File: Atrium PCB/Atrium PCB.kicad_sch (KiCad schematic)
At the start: 167 parts, among them J1 Conn_01x05_Pin, SW1 EC11E09244BS, SW10 SW_Push, SW11 SW_Push, SW12 SW_Push, SW13 SW_Push, SW14 SW_Push, SW15 SW_Push, SW16 SW_Push, SW17 SW_Push, SW18 SW_Push, SW19 SW_Push, SW2 SKRPACE010, SW20 SW_Push, SW21 SW_Push, SW22 SW_Push, SW23 SW_Push, SW24 SW_Push, SW25 SW_Push, SW26 SW_Push, SW27 SW_Push, SW28 SW_Push, SW29 SW_Push, SW3 SKRPACE010, SW30 SW_Push, SW31 SW_Push, SW32 SW_Push, SW33 SW_Push, SW34 SW_Push, SW35 SW_Push, SW36 SW_Push, SW37 SW_Push, SW38 SW_Push, SW39 SW_Push, SW4 SW_Push, SW40 SW_Push, SW41 SW_Push, SW42 SW_Push, SW43 SW_Push, SW44 SW_Push, SW45 SW_Push, SW46 SW_Push, SW47 SW_Push, SW48 SW_Push, SW49 SW_Push, SW5 SW_Push, SW6 SW_Push, SW7 SW_Push, SW8 SW_Push, SW9 SW_Push, U12 AP2112K-3.3, U4 SN74LVC1T45DBVR, X1 X322512MSB4SI

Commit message: sync
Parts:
- removed C44, C46, C47, C48: 100nF, Capacitor_SMD:C_0603_1608Metric, symbol Device:C
- removed C45: 10uF, Capacitor_SMD:C_0805_2012Metric, symbol Device:C
- removed D10, D15, D19, D23, D27, D31, D35, D39, D4: D, symbol Device:D
- removed LED10, LED7, LED8, LED9: SK6812MINI-E_C5149201, easyeda2kicad:LED-SMD_4P-L3.2-W2.8-LS5.9_SK6812MINI-E, symbol easyeda2kicad:SK6812MINI-E_C5149201
- removed R19, R9: 470, Resistor_SMD:R_0603_1608Metric, symbol Device:R
- removed SW12, SW17, SW21, SW25, SW29, SW33, SW37, SW41, SW7: SW_Push, symbol Switch:SW_Push
- removed U4: SN74LVC1T45DBVR, easyeda2kicad:SOT-23-6_L2.9-W1.6-P0.95-LS2.8-BR, symbol easyeda2kicad:SN74LVC1T45DBVR
- added C100, C101, C102, C103, C104, C105, C106, C107, C108, C109, C110, C111, C112, C113, C114, C115, C116, C117, C118, C119, C120, C121, C122, C123, C124, C125, C126, C127, C128, C129, C130, C131, C132, C133, C134, C135, C136, C137, C138, C139, C140, C141, C142, C143, C144, C145, C146, C147, C148, C149, C150, C151, C152, C153, C154, C155, C156, C157, C158, C159, C160, C161, C162, C163, C164, C165, C166, C167, C168, C169, C170, C171, C172, C173, C174, C175, C176, C177, C178, C179, C180, C181, C182, C183, C184, C185, C186, C187, C188, C189, C190, C191, C192, C193, C194, C195, C196, C197, C198, C199, C200, C201, C202, C203, C204, C205, C206, C207, C208, C209, C210, C217, C218, C219, C220, C221, C222, C223, C224, C225, C226, C49, C50, C51, C52, C53, C54, C55, C56, C57, C58, C59, C60, C61, C68, C69, C70, C71, C72, C73, C74, C75, C76, C77, C78, C79, C80, C81, C82, C83, C84, C85, C86, C87, C88, C89, C90, C91, C92, C93, C94, C95, C96, C97, C98, C99: 100nF, Capacitor_SMD:C_0603_1608Metric, symbol Device:C
- added C211, C212, C213, C214, C215, C216: 22uF, Capacitor_SMD:C_0402_1005Metric, symbol Device:C
- added C301, C382, C383, C384, C385, C386, C387: 100nF, Capacitor_SMD:C_0402_1005Metric, symbol Device:C
- added D48, D49, D50, D51, D52: D, symbol Device:D
- added LED175, LED176, LED177, LED178, LED179, LED180, LED181, LED182, LED183, LED184, LED185, LED186, LED187, LED188, LED189, LED190, LED191, LED192, LED193, LED194, LED195, LED196, LED197, LED198, LED199, LED200, LED201, LED202, LED203, LED204, LED205, LED206, LED207, LED208, LED209, LED210, LED211, LED212, LED213, LED214, LED215, LED216, LED217, LED218, LED219, LED220, LED221, LED222, LED223, LED224, LED225, LED226, LED227, LED228, LED229, LED230, LED231, LED232, LED233, LED234, LED235, LED236, LED237, LED238, LED239, LED240, LED241, LED242, LED243, LED244, LED245, LED246, LED247, LED248, LED249, LED250, LED251, LED252, LED253, LED254, LED255, LED256, LED257, LED258, LED259, LED260, LED261, LED262, LED263, LED264, LED265, LED266, LED267, LED268, LED269, LED270, LED271, LED272, LED273, LED274, LED275, LED276, LED277, LED278, LED279, LED280, LED281, LED282, LED283, LED284, LED285, LED286, LED287, LED288, LED289, LED290, LED291, LED292, LED293, LED294, LED295, LED296, LED297, LED298, LED299, LED300, LED301, LED302, LED303, LED304, LED305, LED306, LED307, LED308, LED309, LED310, LED311, LED312, LED313, LED314, LED315, LED316, LED317, LED318, LED319, LED320, LED321, LED322, LED323, LED324, LED325, LED326, LED327, LED328, LED329, LED330, LED331, LED332, LED333, LED334, LED335, LED336, LED337, LED338, LED339, LED340, LED341, LED342: SK6812MINI-E_C5149201, easyeda2kicad:LED-SMD_4P-L3.2-W2.8-LS5.9_SK6812MINI-E, symbol easyeda2kicad:SK6812MINI-E_C5149201
- added R11, R12, R13, R14, R15, R16: 470, Resistor_SMD:R_0603_1608Metric, symbol Device:R
- added SW50, SW51, SW52, SW53, SW54: SW_Push, symbol Switch:SW_Push
- added U1: SN74LVC8T245, symbol Logic_LevelTranslator:SN74LVC8T245
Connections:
- net +5V is gone; now on net GND: C67.2
- net +3.3V: now also U1.1 (V_{CCA}), U1.2 (DIR); no longer C66.2
- net COL_1: now also R11.2, R12.2, R13.2, R14.2, R15.2, R16.2, U1.21 (B1)
- net COL_10: no longer SW45.1
- net COL_2: now also U1.20 (B2)
- net COL_3: now also U1.19 (B3); no longer SW46.1
- net COL_4: now also SW46.1, U1.18 (B4); no longer SW13.1
- net COL_5: now also SW13.1, U1.17 (B5); no longer SW8.1
- net COL_6: now also SW8.1, U1.16 (B6); no longer SW47.1
- net COL_7: now also SW47.1; no longer SW48.1
- net COL_8: now also SW48.1; no longer SW49.1
- net COL_9: now also SW49.1
- net GND: now also C66.2, C100.2, C101.2, C102.2, C103.2, C104.2, C105.2, C106.2, C107.2, C108.2, C109.2, C110.2, C111.2, C112.2, C113.2, C114.2, C115.2, C116.2, C117.2, C118.2, C119.2, C120.2, C121.2, C122.2, C123.2, C124.2, C125.2, C126.2, C127.2, C128.2, C129.2, C130.2, C131.2, C132.2, C133.2, C134.2, C135.2, C136.2, C137.2, C138.2, C139.2, C140.2, C141.2, C142.2, C143.2, C144.2, C145.2, C146.2, C147.2, C148.2, C149.2, C150.2, C151.2, C152.2, C153.2, C154.2, C155.2, C156.2, C157.2, C158.2, C159.2, C160.2, C161.2, C162.2, C163.2, C164.2, C165.2, C166.2, C167.2, C168.2, C169.2, C170.2, C171.2, C172.2, C173.2, C174.2, C175.2, C176.2, C177.2, C178.2, C179.2, C180.2, C181.2, C182.2, C183.2, C184.2, C185.2, C186.2, C187.2, C188.2, C189.2, C190.2, C191.2, C192.2, C193.2, C194.2, C195.2, C196.2, C197.2, C198.2, C199.2, C200.2, C201.2, C202.2, C203.2, C204.2, C205.2, C206.2, C207.2, C208.2, C209.2, C210.2, C211.2, C212.2, C213.2, C214.2, C215.2, C216.2, C217.2, C218.2, C219.2, C220.2, C221.2, C222.2, C223.2, C224.2, C225.2, C226.2, C301.2, C49.2, C50.2, C51.2, C52.2, C53.2, C54.2, C55.2, C56.2, C57.2, C58.2, C59.2, C60.2, C61.2, C68.2, C69.2, C70.2, C71.2, C72.2, C73.2, C74.2, C75.2, C76.2, C77.2, C78.2, C79.2, C80.2, C81.2, C82.2, C83.2, C84.2, C85.2, C86.2, C87.2, C88.2, C89.2, C90.2, C91.2, C92.2, C93.2, C94.2, C95.2, C96.2, C97.2, C98.2, C99.2, LED175.1 (GND), LED176.1 (GND), LED177.1 (GND), LED178.1 (GND), LED179.1 (GND), LED180.1 (GND), LED181.1 (GND), LED182.1 (GND), LED183.1 (GND), LED184.1 (GND), LED185.1 (GND), LED186.1 (GND), LED187.1 (GND), LED188.1 (GND), LED189.1 (GND), LED190.1 (GND), LED191.1 (GND), LED192.1 (GND), LED193.1 (GND), LED194.1 (GND), LED195.1 (GND), LED196.1 (GND), LED197.1 (GND), LED198.1 (GND), LED199.1 (GND), LED200.1 (GND), LED201.1 (GND), LED202.1 (GND), LED203.1 (GND), LED204.1 (GND), LED205.1 (GND), LED206.1 (GND), LED207.1 (GND), LED208.1 (GND), LED209.1 (GND), LED210.1 (GND), LED211.1 (GND), LED212.1 (GND), LED213.1 (GND), LED214.1 (GND), LED215.1 (GND), LED216.1 (GND), LED217.1 (GND), LED218.1 (GND), LED219.1 (GND), LED220.1 (GND), LED221.1 (GND), LED222.1 (GND), LED223.1 (GND), LED224.1 (GND), LED225.1 (GND), LED226.1 (GND), LED227.1 (GND), LED228.1 (GND), LED229.1 (GND), LED230.1 (GND), LED231.1 (GND), LED232.1 (GND), LED233.1 (GND), LED234.1 (GND), LED235.1 (GND), LED236.1 (GND), LED237.1 (GND), LED238.1 (GND), LED239.1 (GND), LED240.1 (GND), LED241.1 (GND), LED242.1 (GND), LED243.1 (GND), LED244.1 (GND), LED245.1 (GND), LED246.1 (GND), LED247.1 (GND), LED248.1 (GND), LED249.1 (GND), LED250.1 (GND), LED251.1 (GND), LED252.1 (GND), LED253.1 (GND), LED254.1 (GND), LED255.1 (GND), LED256.1 (GND), LED257.1 (GND), LED258.1 (GND), LED259.1 (GND), LED260.1 (GND), LED261.1 (GND), LED262.1 (GND), LED263.1 (GND), LED264.1 (GND), LED265.1 (GND), LED266.1 (GND), LED267.1 (GND), LED268.1 (GND), LED269.1 (GND), LED270.1 (GND), LED271.1 (GND), LED272.1 (GND), LED273.1 (GND), LED274.1 (GND), LED275.1 (GND), LED276.1 (GND), LED277.1 (GND), LED278.1 (GND), LED279.1 (GND), LED280.1 (GND), LED281.1 (GND), LED282.1 (GND), LED283.1 (GND), LED284.1 (GND), LED285.1 (GND), LED286.1 (GND), LED287.1 (GND), LED288.1 (GND), LED289.1 (GND), LED290.1 (GND), LED291.1 (GND), LED292.1 (GND), LED293.1 (GND), LED294.1 (GND), LED295.1 (GND), LED296.1 (GND), LED297.1 (GND), LED298.1 (GND), LED299.1 (GND), LED300.1 (GND), LED301.1 (GND), LED302.1 (GND), LED303.1 (GND), LED304.1 (GND), LED305.1 (GND), LED306.1 (GND), LED307.1 (GND), LED308.1 (GND), LED309.1 (GND), LED310.1 (GND), LED311.1 (GND), LED312.1 (GND), LED313.1 (GND), LED314.1 (GND), LED315.1 (GND), LED316.1 (GND), LED317.1 (GND), LED318.1 (GND), LED319.1 (GND), LED320.1 (GND), LED321.1 (GND), LED322.1 (GND), LED323.1 (GND), LED324.1 (GND), LED325.1 (GND), LED326.1 (GND), LED327.1 (GND), LED328.1 (GND), LED329.1 (GND), LED330.1 (GND), LED331.1 (GND), LED332.1 (GND), LED333.1 (GND), LED334.1 (GND), LED335.1 (GND), LED336.1 (GND), LED337.1 (GND), LED338.1 (GND), LED339.1 (GND), LED340.1 (GND), LED341.1 (GND), LED342.1 (GND), U1.10 (A8), U1.11 (GND), U1.12 (GND), U1.13 (GND), U1.22 (~{OE}), U1.9 (A7); no longer C66.1, C67.1
- net ROW_1: now also D43.1 (K), RP2350.16 (GPIO12), D50.1 (K); no longer RP2350.14 (GPIO10)
- net ROW_2: now also RP2350.17 (GPIO13), D48.1 (K), D51.1 (K); no longer RP2350.15 (GPIO11)
- net ROW_3: now also RP2350.18 (GPIO14), D49.1 (K), D52.1 (K); no longer RP2350.16 (GPIO12)
- net ROW_4: now also D11.1 (K), D44.1 (K), D45.1 (K), D46.1 (K), D47.1 (K), D6.1 (K), RP2350.19 (GPIO15); no longer D43.1 (K), RP2350.17 (GPIO13)
- net 5V_A1: now reaches RP2350.27 (GPIO16)
- net 5V_A1: now also U1.3 (A1)
- net 5V_A2: now reaches RP2350.28 (GPIO17)
- net 5V_A2: now also U1.4 (A2)
- net 5V_A3: now reaches RP2350.29 (GPIO18)
- net 5V_A3: now also U1.5 (A3)
- removed net ROW_5: D11.1 (K), D44.1 (K), D45.1 (K), D46.1 (K), D47.1 (K), D6.1 (K), RP2350.18 (GPIO14)
- net RP2350_GPIO_19 renamed 5V_A4
- net 5V_A4: now also U1.6 (A4)
- net RP2350_GPIO_20 renamed 5V_A5
- net 5V_A5: now also U1.7 (A5)
- net RP2350_GPIO_21 renamed 5V_A6
- net 5V_A6: now also U1.8 (A6)
- new net: LED321.2 (DIN), LED328.4 (DOUT)
- new net: LED315.2 (DIN), LED321.4 (DOUT)
- new net: D48.2 (A), SW50.2
- new net: LED302.2 (DIN), LED309.4 (DOUT)
- new net: LED295.2 (DIN), LED302.4 (DOUT)
- new net: LED241.2 (DIN), LED248.4 (DOUT)
- new net: LED234.2 (DIN), LED241.4 (DOUT)
- new net: D49.2 (A), SW51.2
- new net: LED207.4 (DOUT), LED214.2 (DIN)
- new net: LED214.4 (DOUT), LED221.2 (DIN)
- new net: C216.1, C387.2
- new net: LED264.2 (DIN), R14.1
- new net: LED264.4 (DOUT), LED271.2 (DIN)
- new net: LED245.4 (DOUT), LED252.2 (DIN)
- new net: LED252.4 (DOUT), LED253.2 (DIN)
- new net: LED319.4 (DOUT), LED326.2 (DIN)
- new net: LED326.4 (DOUT), LED333.2 (DIN)
- new net: LED305.4 (DOUT), LED312.2 (DIN)
- new net: LED308.4 (DOUT), LED309.2 (DIN)
- new net: LED307.2 (DIN), LED314.4 (DOUT)
- new net: LED300.2 (DIN), LED307.4 (DOUT)
- new net: LED234.4 (DOUT), LED235.2 (DIN)
- new net: LED233.4 (DOUT), LED240.2 (DIN)
- new net: LED240.4 (DOUT), LED247.2 (DIN)
- new net: LED271.4 (DOUT), LED278.2 (DIN)
- new net: LED278.4 (DOUT), LED285.2 (DIN)
- new net: LED285.4 (DOUT), LED286.2 (DIN)
- new net: LED279.2 (DIN), LED286.4 (DOUT)
- new net: LED280.4 (DOUT), LED281.2 (DIN)
- new net: LED274.2 (DIN), LED281.4 (DOUT)
- new net: LED246.2 (DIN), LED253.4 (DOUT)
- new net: LED197.2 (DIN), LED198.4 (DOUT)
- new net: LED196.2 (DIN), LED197.4 (DOUT)
- new net: LED208.2 (DIN), R12.1
- new net: LED206.2 (DIN), LED213.4 (DOUT)
- new net: LED206.4 (DOUT), LED207.2 (DIN)
- new net: LED179.4 (DOUT), LED180.2 (DIN)
- new net: LED180.4 (DOUT), LED181.2 (DIN)
- new net: LED226.4 (DOUT), LED227.2 (DIN)
- new net: LED220.2 (DIN), LED227.4 (DOUT)
- new net: LED188.2 (DIN), LED189.4 (DOUT)
- new net: LED187.2 (DIN), LED188.4 (DOUT)
- new net: LED195.2 (DIN), LED196.4 (DOUT)
- new net: LED195.4 (DOUT), LED199.2 (DIN)
- new net: LED266.4 (DOUT), LED273.2 (DIN)
- new net: LED273.4 (DOUT), LED280.2 (DIN)
- new net: LED324.4 (DOUT), LED331.2 (DIN)
- new net: LED331.4 (DOUT), LED338.2 (DIN)
- new net: LED290.2 (DIN), LED297.4 (DOUT)
- new net: LED290.4 (DOUT), LED291.2 (DIN)
- new net: LED232.2 (DIN), LED239.4 (DOUT)
- new net: LED232.4 (DOUT), LED233.2 (DIN)
- new net: LED259.2 (DIN), LED265.4 (DOUT)
- new net: LED259.4 (DOUT), LED266.2 (DIN)
- new net: LED315.4 (DOUT), LED322.2 (DIN)
- new net: LED322.4 (DOUT), LED329.2 (DIN)
- new net: LED211.2 (DIN), LED218.4 (DOUT)
- new net: LED204.2 (DIN), LED211.4 (DOUT)
- new net: LED200.4 (DOUT), LED201.2 (DIN)
- new net: LED201.4 (DOUT), LED202.2 (DIN)
- new net: LED325.2 (DIN), LED332.4 (DOUT)
- new net: LED318.2 (DIN), LED325.4 (DOUT)
- new net: LED191.4 (DOUT), LED192.2 (DIN)
- new net: LED192.4 (DOUT), LED193.2 (DIN)
- new net: LED329.4 (DOUT), LED336.2 (DIN)
- new net: LED336.4 (DOUT), LED337.2 (DIN)
- new net: LED175.4 (DOUT), LED176.2 (DIN)
- new net: LED176.4 (DOUT), LED177.2 (DIN)
- new net: LED216.2 (DIN), LED223.4 (DOUT)
- new net: LED209.2 (DIN), LED216.4 (DOUT)
- new net: LED177.4 (DOUT), LED178.2 (DIN)
- new net: LED178.4 (DOUT), LED179.2 (DIN)
- new net: LED184.4 (DOUT), LED185.2 (DIN)
- new net: LED185.4 (DOUT), LED186.2 (DIN)
- new net: LED213.2 (DIN), LED220.4 (DOUT)
- new net: LED262.2 (DIN), LED269.4 (DOUT)
- new net: LED262.4 (DOUT), LED263.2 (DIN)
- new net: LED296.4 (DOUT), LED303.2 (DIN)
- new net: LED303.4 (DOUT), LED310.2 (DIN)
- new net: LED267.2 (DIN), LED274.4 (DOUT)
- new net: C212.1, C383.2
- new net: LED304.2 (DIN), LED311.4 (DOUT)
- new net: LED297.2 (DIN), LED304.4 (DOUT)
- new net: LED203.4 (DOUT), LED210.2 (DIN)
- new net: LED210.4 (DOUT), LED217.2 (DIN)
- new net: LED333.4 (DOUT), LED340.2 (DIN)
- new net: LED291.4 (DOUT), LED298.2 (DIN)
- new net: LED248.2 (DIN), LED255.4 (DOUT)
- new net: LED175.2 (DIN), R11.1
- new net: LED334.4 (DOUT), LED341.2 (DIN)
- new net: LED341.4 (DOUT), LED342.2 (DIN)
- new net: LED338.4 (DOUT), LED339.2 (DIN)
- new net: LED239.2 (DIN), LED246.4 (DOUT)
- new net: LED260.2 (DIN), LED267.4 (DOUT)
- new net: LED260.4 (DOUT), LED261.2 (DIN)
- new net: C214.1, C385.2
- new net: LED243.4 (DOUT), LED250.2 (DIN)
- new net: LED250.4 (DOUT), LED257.2 (DIN)
- new net: LED194.4 (DOUT), LED198.2 (DIN)
- new net: D51.2 (A), SW53.2
- new net: LED292.4 (DOUT), LED299.2 (DIN)
- new net: LED299.4 (DOUT), LED306.2 (DIN)
- new net: LED189.2 (DIN), LED190.4 (DOUT)
- new net: LED186.4 (DOUT), LED190.2 (DIN)
- new net: LED236.2 (DIN), R13.1
- new net: LED236.4 (DOUT), LED243.2 (DIN)
- new net: D52.2 (A), SW54.2
- new net: LED298.4 (DOUT), LED305.2 (DIN)
- new net: LED208.4 (DOUT), LED215.2 (DIN)
- new net: LED263.4 (DOUT), LED270.2 (DIN)
- new net: LED235.4 (DOUT), LED242.2 (DIN)
- new net: C211.1, C382.2
- new net: LED218.2 (DIN), LED225.4 (DOUT)
- new net: LED247.4 (DOUT), LED254.2 (DIN)
- new net: LED254.4 (DOUT), LED255.2 (DIN)
- new net: LED251.2 (DIN), LED258.4 (DOUT)
- new net: LED244.2 (DIN), LED251.4 (DOUT)
- new net: LED306.4 (DOUT), LED313.2 (DIN)
- new net: LED313.4 (DOUT), LED314.2 (DIN)
- new net: LED270.4 (DOUT), LED277.2 (DIN)
- new net: LED199.4 (DOUT), LED200.2 (DIN)
- new net: LED332.2 (DIN), LED339.4 (DOUT)
- new net: LED328.2 (DIN), LED335.4 (DOUT)
- new net: LED187.4 (DOUT), LED191.2 (DIN)
- new net: LED317.4 (DOUT), LED324.2 (DIN)
- new net: LED183.4 (DOUT), LED184.2 (DIN)
- new net: LED293.2 (DIN), LED300.4 (DOUT)
- new net: LED287.2 (DIN), LED293.4 (DOUT)
- new net: C213.1, C384.2
- new net: LED272.2 (DIN), LED279.4 (DOUT)
- new net: LED181.4 (DOUT), LED182.2 (DIN)
- new net: LED277.4 (DOUT), LED284.2 (DIN)
- new net: LED320.2 (DIN), R16.1
- new net: LED320.4 (DOUT), LED327.2 (DIN)
- new net: LED330.2 (DIN), LED337.4 (DOUT)
- new net: LED323.2 (DIN), LED330.4 (DOUT)
- new net: LED282.4 (DOUT), LED283.2 (DIN)
- new net: LED276.2 (DIN), LED283.4 (DOUT)
- new net: LED310.4 (DOUT), LED311.2 (DIN)
- new net: LED242.4 (DOUT), LED249.2 (DIN)
- new net: LED249.4 (DOUT), LED256.2 (DIN)
- new net: LED217.4 (DOUT), LED224.2 (DIN)
- new net: LED182.4 (DOUT), LED183.2 (DIN)
- new net: D50.2 (A), SW52.2
- new net: LED269.2 (DIN), LED276.4 (DOUT)
- new net: LED224.4 (DOUT), LED225.2 (DIN)
- new net: LED221.4 (DOUT), LED228.2 (DIN)
- new net: LED288.2 (DIN), LED295.4 (DOUT)
- new net: LED288.4 (DOUT), LED289.2 (DIN)
- new net: LED265.2 (DIN), LED272.4 (DOUT)
- new net: LED289.4 (DOUT), LED296.2 (DIN)
- new net: LED316.2 (DIN), LED323.4 (DOUT)
- new net: LED316.4 (DOUT), LED317.2 (DIN)
- new net: LED203.2 (DIN), LED209.4 (DOUT)
- new net: LED219.4 (DOUT), LED226.2 (DIN)
- new net: LED327.4 (DOUT), LED334.2 (DIN)
- new net: LED257.4 (DOUT), LED258.2 (DIN)
- new net: LED215.4 (DOUT), LED222.2 (DIN)
- new net: LED222.4 (DOUT), LED229.2 (DIN)
- new net: LED261.4 (DOUT), LED268.2 (DIN)
- new net: LED268.4 (DOUT), LED275.2 (DIN)
- new net: LED205.4 (DOUT), LED212.2 (DIN)
- new net: LED212.4 (DOUT), LED219.2 (DIN)
- new net: LED231.2 (DIN), LED237.4 (DOUT)
- new net: LED231.4 (DOUT), LED238.2 (DIN)
- new net: LED292.2 (DIN), R15.1
- new net: LED301.4 (DOUT), LED308.2 (DIN)
- new net: LED238.4 (DOUT), LED245.2 (DIN)
- new net: LED229.4 (DOUT), LED230.2 (DIN)
- new net: C215.1, C386.2
- new net: LED223.2 (DIN), LED230.4 (DOUT)
- new net: LED275.4 (DOUT), LED282.2 (DIN)
- new net: LED204.4 (DOUT), LED205.2 (DIN)
- new net: LED318.4 (DOUT), LED319.2 (DIN)
- new net: LED193.4 (DOUT), LED194.2 (DIN)
- new net: LED287.4 (DOUT), LED294.2 (DIN)
- new net: LED237.2 (DIN), LED244.4 (DOUT)
- new net: LED335.2 (DIN), LED342.4 (DOUT)
- new net: LED294.4 (DOUT), LED301.2 (DIN)
- new net +5V_LED: C100.1, C101.1, C102.1, C103.1, C104.1, C105.1, C106.1, C107.1, C108.1, C109.1, C110.1, C111.1, C112.1, C113.1, C114.1, C115.1, C116.1, C117.1, C118.1, C119.1, C120.1, C121.1, C122.1, C123.1, C124.1, C125.1, C126.1, C127.1, C128.1, C129.1, C130.1, C131.1, C132.1, C133.1, C134.1, C135.1, C136.1, C137.1, C138.1, C139.1, C140.1, C141.1, C142.1, C143.1, C144.1, C145.1, C146.1, C147.1, C148.1, C149.1, C150.1, C151.1, C152.1, C153.1, C154.1, C155.1, C156.1, C157.1, C158.1, C159.1, C160.1, C161.1, C162.1, C163.1, C164.1, C165.1, C166.1, C167.1, C168.1, C169.1, C170.1, C171.1, C172.1, C173.1, C174.1, C175.1, C176.1, C177.1, C178.1, C179.1, C180.1, C181.1, C182.1, C183.1, C184.1, C185.1, C186.1, C187.1, C188.1, C189.1, C190.1, C191.1, C192.1, C193.1, C194.1, C195.1, C196.1, C197.1, C198.1, C199.1, C200.1, C201.1, C202.1, C203.1, C204.1, C205.1, C206.1, C207.1, C208.1, C209.1, C210.1, C217.1, C218.1, C219.1, C220.1, C221.1, C222.1, C223.1, C224.1, C225.1, C226.1, C301.1, C382.1, C383.1, C384.1, C385.1, C386.1, C387.1, C49.1, C50.1, C51.1, C52.1, C53.1, C54.1, C55.1, C56.1, C57.1, C58.1, C59.1, C60.1, C61.1, C66.1, C67.1, C68.1, C69.1, C70.1, C71.1, C72.1, C73.1, C74.1, C75.1, C76.1, C77.1, C78.1, C79.1, C80.1, C81.1, C82.1, C83.1, C84.1, C85.1, C86.1, C87.1, C88.1, C89.1, C90.1, C91.1, C92.1, C93.1, C94.1, C95.1, C96.1, C97.1, C98.1, C99.1, LED175.3 (VDD), LED176.3 (VDD), LED177.3 (VDD), LED178.3 (VDD), LED179.3 (VDD), LED180.3 (VDD), LED181.3 (VDD), LED182.3 (VDD), LED183.3 (VDD), LED184.3 (VDD), LED185.3 (VDD), LED186.3 (VDD), LED188.3 (VDD), LED189.3 (VDD), LED190.3 (VDD), LED191.3 (VDD), LED192.3 (VDD), LED193.3 (VDD), LED194.3 (VDD), LED195.3 (VDD), LED196.3 (VDD), LED197.3 (VDD), LED198.3 (VDD), LED199.3 (VDD), LED200.3 (VDD), LED201.3 (VDD), LED202.3 (VDD), LED203.3 (VDD), LED205.3 (VDD), LED206.3 (VDD), LED207.3 (VDD), LED208.3 (VDD), LED209.3 (VDD), LED210.3 (VDD), LED211.3 (VDD), LED212.3 (VDD), LED213.3 (VDD), LED214.3 (VDD), LED215.3 (VDD), LED216.3 (VDD), LED217.3 (VDD), LED218.3 (VDD), LED219.3 (VDD), LED220.3 (VDD), LED221.3 (VDD), LED222.3 (VDD), LED223.3 (VDD), LED224.3 (VDD), LED225.3 (VDD), LED226.3 (VDD), LED227.3 (VDD), LED228.3 (VDD), LED229.3 (VDD), LED230.3 (VDD), LED231.3 (VDD), LED233.3 (VDD), LED234.3 (VDD), LED235.3 (VDD), LED236.3 (VDD), LED237.3 (VDD), LED238.3 (VDD), LED239.3 (VDD), LED240.3 (VDD), LED241.3 (VDD), LED242.3 (VDD), LED243.3 (VDD), LED244.3 (VDD), LED245.3 (VDD), LED246.3 (VDD), LED247.3 (VDD), LED248.3 (VDD), LED249.3 (VDD), LED250.3 (VDD), LED251.3 (VDD), LED252.3 (VDD), LED253.3 (VDD), LED254.3 (VDD), LED255.3 (VDD), LED256.3 (VDD), LED257.3 (VDD), LED258.3 (VDD), LED259.3 (VDD), LED261.3 (VDD), LED262.3 (VDD), LED263.3 (VDD), LED264.3 (VDD), LED265.3 (VDD), LED266.3 (VDD), LED267.3 (VDD), LED268.3 (VDD), LED269.3 (VDD), LED270.3 (VDD), LED271.3 (VDD), LED272.3 (VDD), LED273.3 (VDD), LED274.3 (VDD), LED275.3 (VDD), LED276.3 (VDD), LED277.3 (VDD), LED278.3 (VDD), LED279.3 (VDD), LED280.3 (VDD), LED281.3 (VDD), LED282.3 (VDD), LED283.3 (VDD), LED284.3 (VDD), LED285.3 (VDD), LED286.3 (VDD), LED287.3 (VDD), LED289.3 (VDD), LED290.3 (VDD), LED291.3 (VDD), LED292.3 (VDD), LED293.3 (VDD), LED294.3 (VDD), LED295.3 (VDD), LED296.3 (VDD), LED297.3 (VDD), LED298.3 (VDD), LED299.3 (VDD), LED300.3 (VDD), LED301.3 (VDD), LED302.3 (VDD), LED303.3 (VDD), LED304.3 (VDD), LED305.3 (VDD), LED306.3 (VDD), LED307.3 (VDD), LED308.3 (VDD), LED309.3 (VDD), LED310.3 (VDD), LED311.3 (VDD), LED312.3 (VDD), LED313.3 (VDD), LED314.3 (VDD), LED315.3 (VDD), LED317.3 (VDD), LED318.3 (VDD), LED319.3 (VDD), LED320.3 (VDD), LED321.3 (VDD), LED322.3 (VDD), LED323.3 (VDD), LED324.3 (VDD), LED325.3 (VDD), LED326.3 (VDD), LED327.3 (VDD), LED328.3 (VDD), LED329.3 (VDD), LED330.3 (VDD), LED331.3 (VDD), LED332.3 (VDD), LED333.3 (VDD), LED334.3 (VDD), LED335.3 (VDD), LED336.3 (VDD), LED337.3 (VDD), LED338.3 (VDD), LED339.3 (VDD), LED340.3 (VDD), LED341.3 (VDD), LED342.3 (VDD), U1.23 (V_{CCB}), U1.24 (V_{CCB})
- new net COL_11: RP2350.14 (GPIO10), SW45.1, SW50.1, SW51.1
- new net COL_12: RP2350.15 (GPIO11), SW52.1, SW53.1, SW54.1
- no-connect marks 10 -> 12
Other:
- note added: "COL_1"
- note added: "COL_2"
- note added: "COL_3"
- note added: "COL_4"
- note added: "COL_5"
- note added: "COL_6"
- note added: "Cirque Trackball"
- note removed: "LED ARRAY"
- moved on the sheet: C65, D11, D44, D45, D46, D47, D6, SW1, SW13, SW46, SW47, SW48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

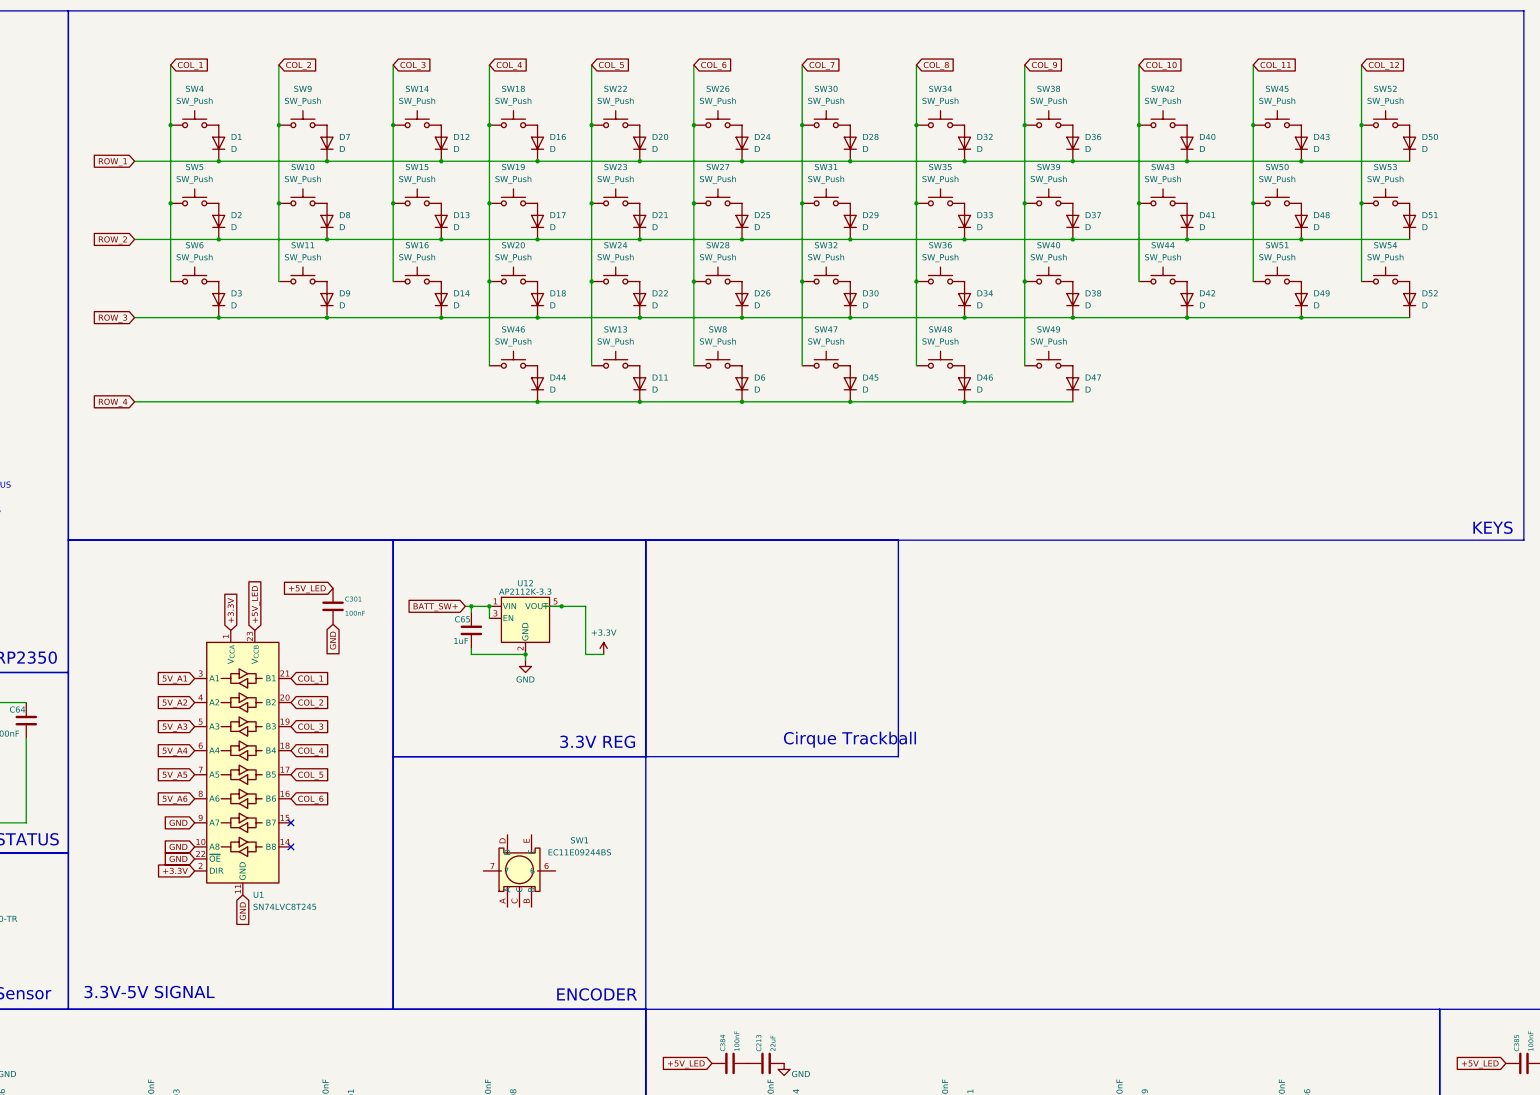
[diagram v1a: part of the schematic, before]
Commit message: sync
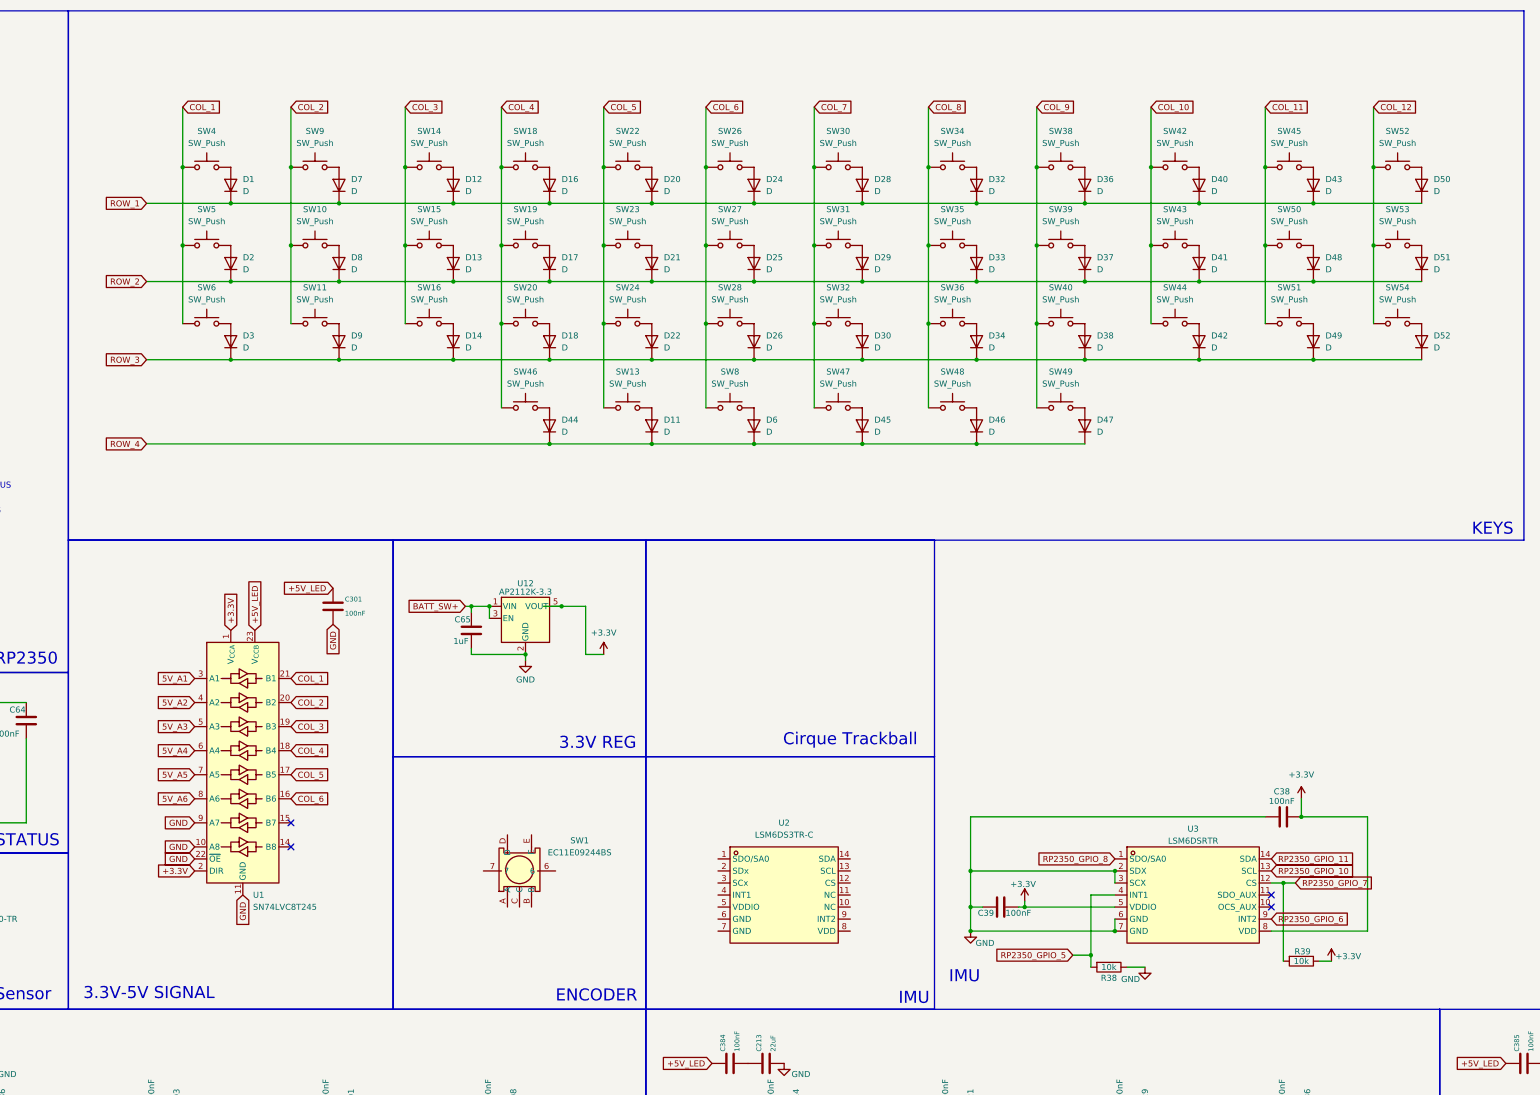
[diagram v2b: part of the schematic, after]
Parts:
- added C38, C39: 100nF, Capacitor_SMD:C_0603_1608Metric, symbol Device:C
- added R38, R39: 10k, Resistor_SMD:R_0603_1608Metric, symbol Device:R
- added U2: LSM6DS3TR-C, easyeda2kicad:LGA-14_L3.0-W2.5-P0.50-TL, symbol easyeda2kicad:LSM6DS3TR-C
- added U3: LSM6DSRTR, easyeda2kicad:LGA-14_L3.0-W2.5-P0.50-BR, symbol easyeda2kicad:LSM6DSRTR
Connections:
- net +3.3V: now also C38.1, C39.1, R39.1, U3.5 (VDDIO), U3.8 (VDD)
- net GND: now also C38.2, C39.2, R38.1, U3.2 (SDX), U3.3 (SCX), U3.6 (GND), U3.7 (GND)
- new net RP2350_GPIO_10: U3.13 (SCL)
- new net RP2350_GPIO_11: U3.14 (SDA)
- new net RP2350_GPIO_5: R38.2, U3.4 (INT1)
- new net RP2350_GPIO_6: U3.9 (INT2)
- new net RP2350_GPIO_7: R39.2, U3.12 (CS)
- new net RP2350_GPIO_8: U3.1 (SDO/SA0)
- no-connect marks 12 -> 14
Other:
- note added: "IMU"
- moved on the sheet: D1, D11, D12, D13, D14, D16, D17, D18, D2, D20, D21, D22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
